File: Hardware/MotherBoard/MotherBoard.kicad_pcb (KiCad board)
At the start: 2 copper layers, 145 x 160 mm, 55 parts, among them J1 POWER, J10 I/O_PWR, J11 DMA_PULLUP, J12 NMI_PULLUP, J13 USB_OTG, J14 IRQ0_PULLUP, J2 I/O0, J3 ISA1, J4 ISA0, J5 I/O1, J6 EXTRN_CLCK, J9 Conn_02x02_Odd_Even, SW1 RESET_SW, SW2 ON_OFF, U1 AMS1117-5.0, U10 74HC245, U11 74HC245, U12 74HC245, U13 74HC541, U14 74HC541, U2 AT28C256, U3 WD65C22, U4 AS6C62256, U5 WD65C02, U6 74HC148, U7 74HC574, U8 ATF22V10B, U9 74HC245, X1 ACO-1MHz

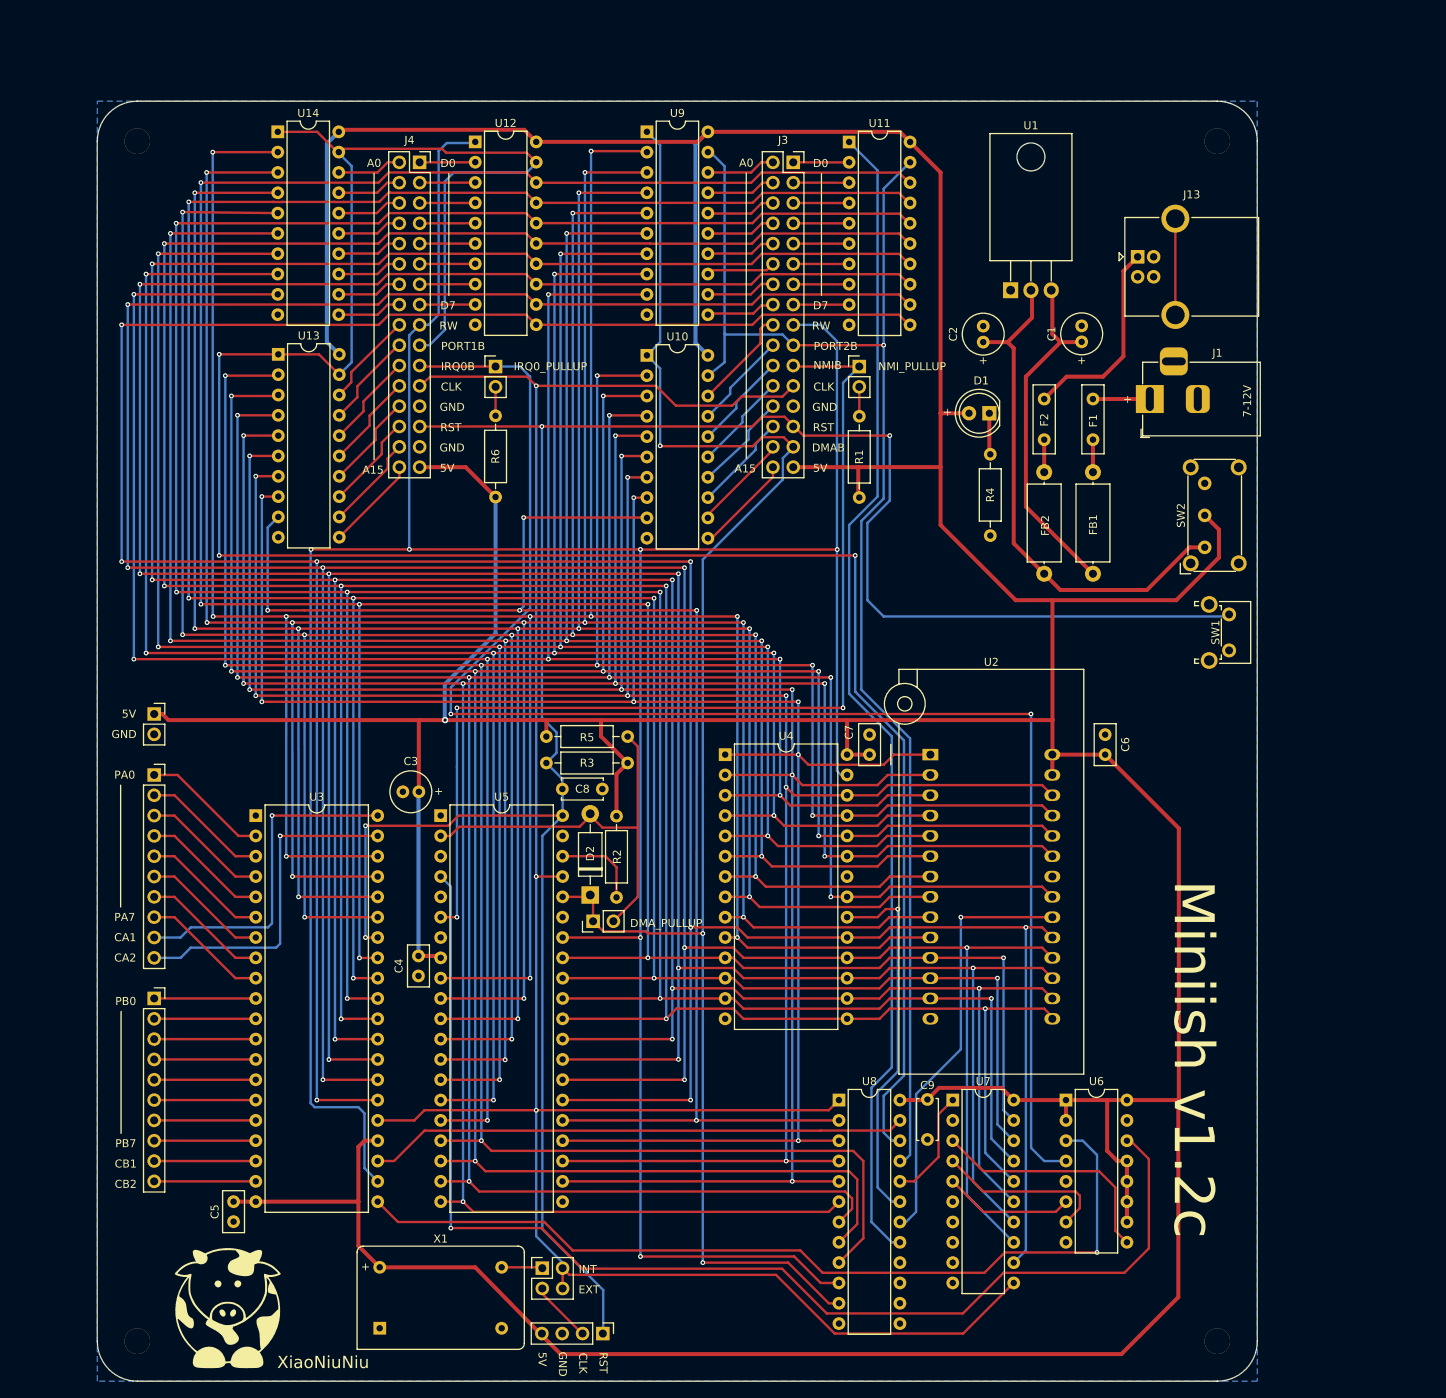
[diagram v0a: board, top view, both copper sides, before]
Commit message: New motherboard version
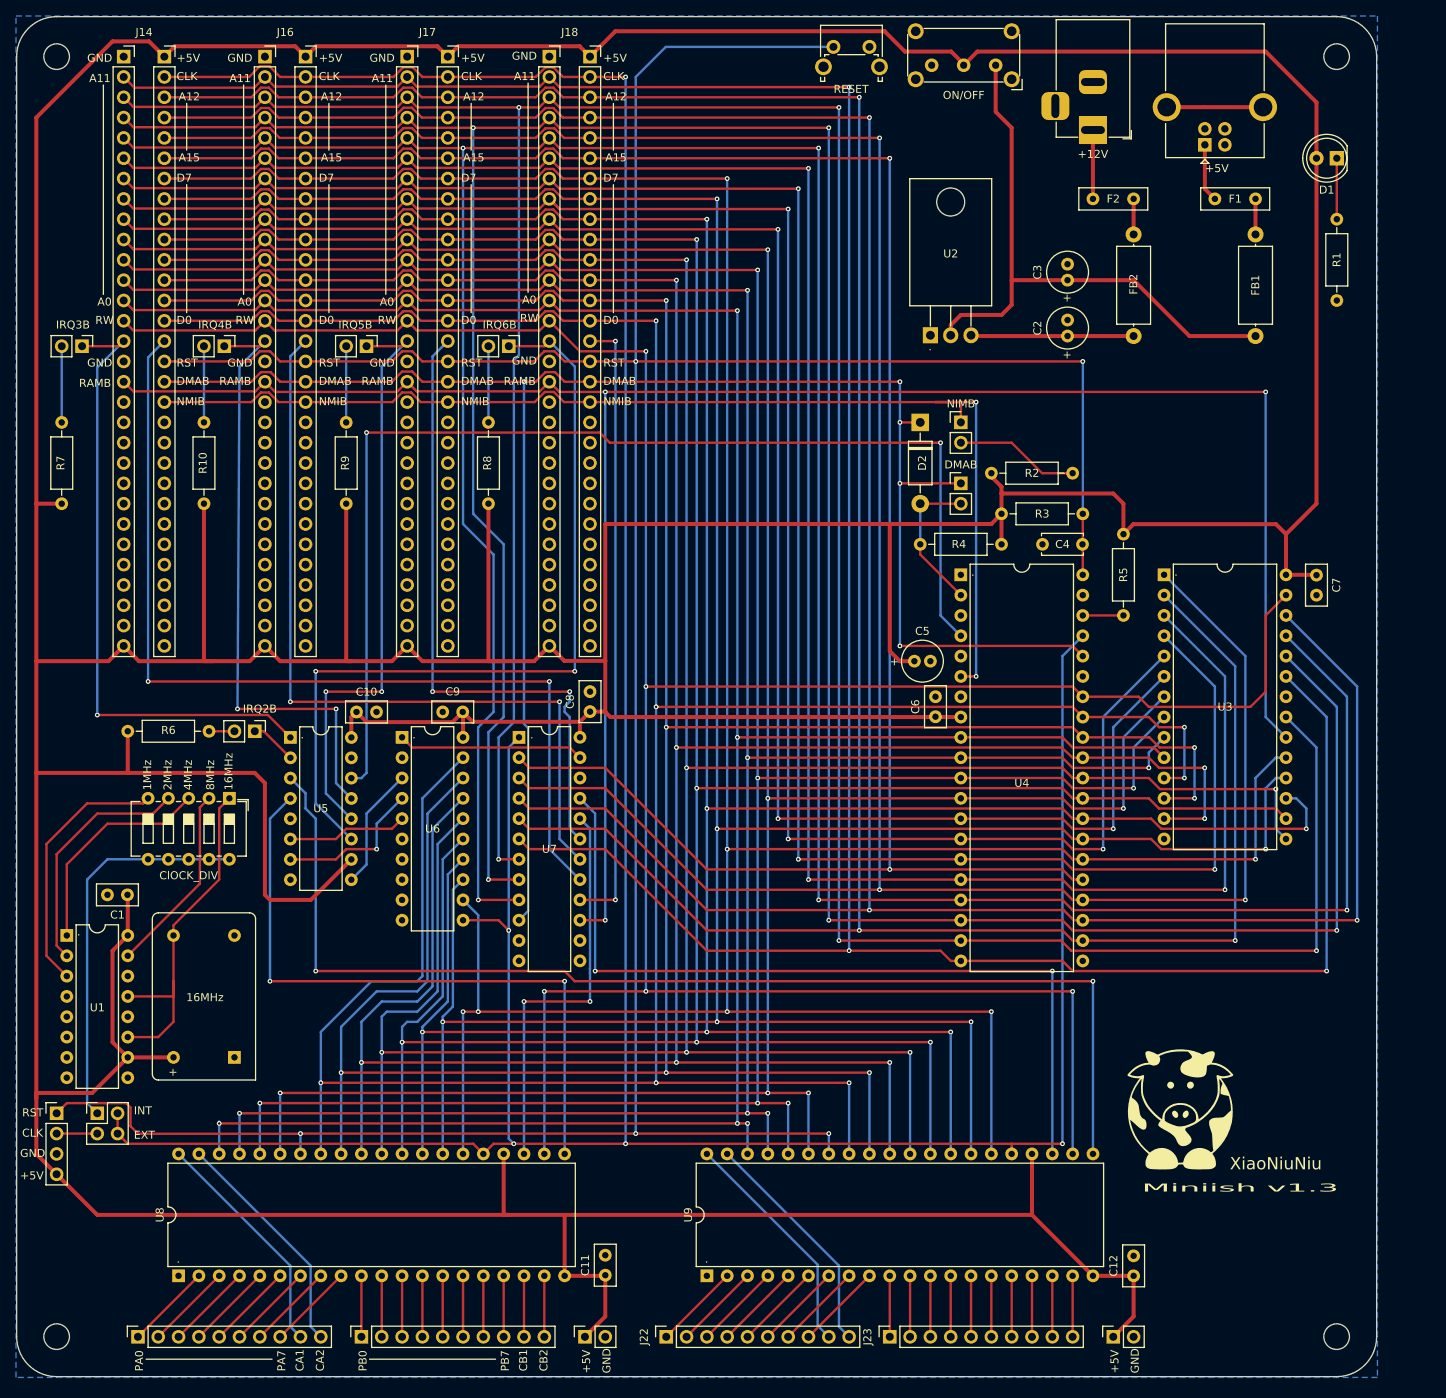
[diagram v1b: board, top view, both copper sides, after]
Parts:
- removed J1: POWER, Connector_BarrelJack:BarrelJack_Horizontal
- removed J10: I/O_PWR, Connector_PinSocket_2.54mm:PinSocket_1x02_P2.54mm_Vertical
- removed J11: DMA_PULLUP, Connector_PinHeader_2.54mm:PinHeader_1x02_P2.54mm_Vertical
- removed J12: NMI_PULLUP, Connector_PinHeader_2.54mm:PinHeader_1x02_P2.54mm_Vertical
- removed J13: USB_OTG, Connector_USB:USB_B_OST_USB-B1HSxx_Horizontal
- removed J2: I/O0, Connector_PinSocket_2.54mm:PinSocket_1x10_P2.54mm_Vertical
- removed J5: I/O1, Connector_PinSocket_2.54mm:PinSocket_1x10_P2.54mm_Vertical
- removed J6: EXTRN_CLCK, Connector_PinHeader_2.54mm:PinHeader_1x04_P2.54mm_Vertical
- removed J9: Conn_02x02_Odd_Even, Connector_PinHeader_2.54mm:PinHeader_2x02_P2.54mm_Vertical
- removed SW1: RESET_SW, Button_Switch_THT:SW_Tactile_SPST_Angled_PTS645Vx83-2LFS
- removed SW2: ON_OFF, Button_Switch_THT:SW_E-Switch_EG1224_SPDT_Angled
- removed U10, U11, U12: 74HC245, Package_DIP:DIP-20_W7.62mm
- removed U13, U14: 74HC541, Package_DIP:DIP-20_W7.62mm
- removed X1: ACO-1MHz, Oscillator:Oscillator_DIP-14
- removed the XiaoNiuNiu at (39.5, 176.1)
- added +12V: POWER, Connector_BarrelJack:BarrelJack_Horizontal, F.Cu at (147.7, 28.8)
- added +5V: USB_OTG, Connector_USB:USB_B_OST_USB-B1HSxx_Horizontal, F.Cu at (161.6, 30.7)
- added 16MHz: ACO-16MHz, Oscillator:Oscillator_DIP-14, F.Cu at (40.3, 144.7)
- added C10: 100nF, Capacitor_THT:C_Disc_D5.0mm_W2.5mm_P2.50mm, F.Cu at (55.6, 101.6)
- added C11: 100nF, Capacitor_THT:C_Disc_D5.0mm_W2.5mm_P2.50mm, F.Cu at (86.7, 172.0)
- added C12: 100nF, Capacitor_THT:C_Disc_D5.0mm_W2.5mm_P2.50mm, F.Cu at (152.7, 172.0)
- added ClOCK_DIV: CLOCK_DIV, Button_Switch_THT:SW_DIP_SPSTx05_Slide_6.7x14.26mm_W7.62mm_P2.54mm_LowProfile, F.Cu at (39.7, 112.4)
- added DMAB: DMA_PULLUP, Connector_PinHeader_2.54mm:PinHeader_1x02_P2.54mm_Vertical, F.Cu at (131.1, 73.0)
- added IRQ2B: IRQ2_PULLUP, Connector_PinHeader_2.54mm:PinHeader_1x02_P2.54mm_Vertical, F.Cu at (42.9, 104.0)
- added IRQ3B: IRQ3_PULLUP, Connector_PinHeader_2.54mm:PinHeader_1x02_P2.54mm_Vertical, F.Cu at (21.3, 55.8)
- added IRQ4B: IRQ4_PULLUP, Connector_PinHeader_2.54mm:PinHeader_1x02_P2.54mm_Vertical, F.Cu at (39.1, 55.8)
- added IRQ5B: IRQ5_PULLUP, Connector_PinHeader_2.54mm:PinHeader_1x02_P2.54mm_Vertical, F.Cu at (56.8, 55.8)
- added IRQ6B: IRQ6_PULLUP, Connector_PinHeader_2.54mm:PinHeader_1x02_P2.54mm_Vertical, F.Cu at (74.6, 55.8)
- added J16: PORT2, NESConnector:NES_Cartdrige, F.Cu at (46.7, 56.5)
- added J17: PORT2, NESConnector:NES_Cartdrige, F.Cu at (64.5, 56.5)
- added J18: PORT3, NESConnector:NES_Cartdrige, F.Cu at (82.2, 56.5)
- added J19: GPIO1, Connector_PinSocket_2.54mm:PinSocket_1x10_P2.54mm_Vertical, F.Cu at (28.3, 179.7)
- added J20: GPIO2, Connector_PinSocket_2.54mm:PinSocket_1x10_P2.54mm_Vertical, F.Cu at (56.2, 179.7)
- added J21: GPIO1_PWR, Connector_PinSocket_2.54mm:PinSocket_1x02_P2.54mm_Vertical, F.Cu at (84.2, 179.7)
- added J22: GPIO3, Connector_PinSocket_2.54mm:PinSocket_1x10_P2.54mm_Vertical, F.Cu at (94.3, 179.7)
- added J23: GPIO4, Connector_PinSocket_2.54mm:PinSocket_1x10_P2.54mm_Vertical, F.Cu at (122.2, 179.7)
- added J24: GPIO2_PWR, Connector_PinSocket_2.54mm:PinSocket_1x02_P2.54mm_Vertical, F.Cu at (150.2, 179.7)
- added NIMB: NMI_PULLUP, Connector_PinHeader_2.54mm:PinHeader_1x02_P2.54mm_Vertical, F.Cu at (131.1, 65.4)
- added ON/OFF: ON_OFF, Button_Switch_THT:SW_E-Switch_EG1224_SPDT_Angled, F.Cu at (135.5, 20.7)
- added R10: 3K3, Resistor_THT:R_Axial_DIN0207_L6.3mm_D2.5mm_P10.16mm_Horizontal, F.Cu at (36.5, 65.4)
- added R7: 3K3, Resistor_THT:R_Axial_DIN0207_L6.3mm_D2.5mm_P10.16mm_Horizontal, F.Cu at (18.7, 65.4)
- added R8: 3K3, Resistor_THT:R_Axial_DIN0207_L6.3mm_D2.5mm_P10.16mm_Horizontal, F.Cu at (72.1, 65.4)
- added R9: 3K3, Resistor_THT:R_Axial_DIN0207_L6.3mm_D2.5mm_P10.16mm_Horizontal, F.Cu at (54.3, 65.4)
- added RESET: RESET_SW, Button_Switch_THT:SW_Tactile_SPST_Angled_PTS645Vx83-2LFS, F.Cu at (115.2, 18.4)
- added XiaoNiuNiu: LOGO, Cow:SmallCow, F.Cu at (158.6, 151.2)
- C1: value 10uF -> 10nF; footprint Capacitor_THT:C_Radial_D5.0mm_H11.0mm_P2.00mm -> Capacitor_THT:C_Disc_D5.0mm_W2.5mm_P2.50mm
- C2: value 22uF -> 10uF
- C3: value 10uF -> 22uF
- C4: value 100nF -> 470nF; footprint Capacitor_THT:C_Disc_D5.0mm_W2.5mm_P2.50mm -> Capacitor_THT:C_Disc_D5.0mm_W2.5mm_P5.00mm
- C5: value 100nF -> 10uF; footprint Capacitor_THT:C_Disc_D5.0mm_W2.5mm_P2.50mm -> Capacitor_THT:C_Radial_D5.0mm_H11.0mm_P2.00mm
- C8: value 470nF -> 220nF; footprint Capacitor_THT:C_Disc_D5.0mm_W2.5mm_P5.00mm -> Capacitor_THT:C_Disc_D5.0mm_W2.5mm_P2.50mm
- C9: value 220nF -> 100nF; footprint Capacitor_THT:C_Disc_D5.0mm_W2.5mm_P5.00mm -> Capacitor_THT:C_Disc_D5.0mm_W2.5mm_P2.50mm
- J14: value IRQ0_PULLUP -> PORT1; footprint Connector_PinHeader_2.54mm:PinHeader_1x02_P2.54mm_Vertical -> NESConnector:NES_Cartdrige
- J3: value ISA1 -> CLOCK_SEL; footprint Connector_PinSocket_2.54mm:PinSocket_2x16_P2.54mm_Vertical -> Connector_PinHeader_2.54mm:PinHeader_2x02_P2.54mm_Vertical
- J4: value ISA0 -> EXTRN_CLCK; footprint Connector_PinSocket_2.54mm:PinSocket_2x16_P2.54mm_Vertical -> Connector_PinHeader_2.54mm:PinHeader_1x04_P2.54mm_Vertical
- R1: value 3K3 -> 220
- R4: value 220 -> 3K3
- U1: value AMS1117-5.0 -> 74HC590A; footprint Package_TO_SOT_THT:TO-220-3_Horizontal_TabDown -> Package_DIP:DIP-16_W7.62mm
- U2: value AT28C256 -> AMS1117-5.0; footprint Socket:DIP_Socket-28_W11.9_W12.7_W15.24_W17.78_W18.5_3M_228-1277-00-0602J -> Package_TO_SOT_THT:TO-220-3_Horizontal_TabDown
- U3: value WD65C22 -> AS6C62256; footprint Package_DIP:DIP-40_W15.24mm -> Package_DIP:DIP-28_W15.24mm
- U4: value AS6C62256 -> WD65C02; footprint Package_DIP:DIP-28_W15.24mm -> Package_DIP:DIP-40_W15.24mm
- U5: value WD65C02 -> 74HC148; footprint Package_DIP:DIP-40_W15.24mm -> Package_DIP:DIP-16_W7.62mm
- U6: value 74HC148 -> 74HC574; footprint Package_DIP:DIP-16_W7.62mm -> Package_DIP:DIP-20_W7.62mm
- U7: value 74HC574 -> ATF22V10B; footprint Package_DIP:DIP-20_W7.62mm -> Package_DIP:DIP-24_W7.62mm
- U8: value ATF22V10B -> WD65C22; footprint Package_DIP:DIP-24_W7.62mm -> Package_DIP:DIP-40_W15.24mm
- U9: value 74HC245 -> WD65C22; footprint Package_DIP:DIP-20_W7.62mm -> Package_DIP:DIP-40_W15.24mm
- moved H2 150.3 mm to (178.1, 19.6)
- moved H3 149.9 mm to (178.1, 179.6)
- moved J3 147.3 mm to (23.2, 151.7)
- moved H1 145.5 mm to (18.1, 19.6)
- moved H4 145.1 mm to (18.1, 179.6)
- moved U9 143.2 mm to (99.4, 172.0), turned to 90 degrees
- moved U1 142.9 mm to (19.4, 129.5)
- moved C1 137.9 mm to (27.0, 124.4), turned to 180 degrees
- moved J4 127.2 mm to (18.1, 151.7)
- moved U3 117.5 mm to (156.5, 84.4)
- moved C5 108.7 mm to (125.3, 95.2), turned to 0 degrees
- moved C3 103.3 mm to (144.5, 47.6), turned to 90 degrees
- moved C4 97.7 mm to (146.3, 80.6), turned to 180 degrees
- moved U6 94.6 mm to (61.3, 104.7)
- moved U8 85.4 mm to (33.4, 172.0), turned to 90 degrees
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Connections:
- C1 pad 1: Net-(C1-Pad1) -> +5V
- C2 pad 1: Net-(C2-Pad1) -> Net-(#FLG01-pwr)
- C3 pad 1: +5V -> Net-(SW2-A)
- C4 pad 1: +5V -> RESET
- C8 pad 1: RESET -> +5V
- D1 pad 1: Net-(D1-Pad1) -> Net-(D1-K)
- D2 pad 1: /Main /DMAB -> /North Bridge/DMAB
- D2 pad 2: /Main /RDY -> /North Bridge/RDY
- FB1 pad 2: Net-(C1-Pad1) -> Net-(SW2-A)
- FB2 pad 2: Net-(C2-Pad1) -> Net-(#FLG01-pwr)
- J14 pad 1: /North Bridge/IRQ0B -> GND
- J14 pad 2: Net-(J14-Pad2) -> +5V
- J3 pad 2: Net-(J3-Pad2) -> CLOCK
- J3 pad 3: Net-(J3-Pad3) -> ECLOCK
- J3 pad 4: Net-(J3-Pad4) -> CLOCK
- J4 pad 1: Net-(J4-Pad1) -> RESET
- J4 pad 2: Net-(J4-Pad2) -> ECLOCK
- J4 pad 3: Net-(J4-Pad3) -> GND
- J4 pad 4: Net-(J4-Pad4) -> +5V
- R1 pad 1: Net-(J12-Pad2) -> Net-(D1-K)
- R1 pad 2: +5V -> GND
- R2 pad 1: +5V -> Net-(J5-Pin_2)
- R2 pad 2: Net-(R2-Pad2) -> +5V
- R4 pad 1: Net-(D1-Pad1) -> /North Bridge/RDY
- R4 pad 2: GND -> +5V
- R5 pad 1: /Main /RDY -> +5V
- R5 pad 2: +5V -> /North Bridge/SOB
- R6 pad 1: Net-(J14-Pad2) -> Net-(J7-Pin_2)
- U1 pad 1: GND -> /4MHz
- U1 pad 2: Net-(C2-Pad1) -> /2MHz
- U1 pad 3: Net-(C1-Pad1) -> /1MHz
- U2 pad 1: /A14 -> GND
- U2 pad 2: /A12 -> Net-(SW2-A)
- U2 pad 3: /A7 -> Net-(#FLG01-pwr)
- U3 pad 1: GND -> /GPIO/A14
- U3 pad 10: PB0 -> /GPIO/A0
- U3 pad 11: PB1 -> /GPIO/D0
- U3 pad 12: PB2 -> /GPIO/D1
- U3 pad 13: PB3 -> /GPIO/D2
- U3 pad 14: PB4 -> GND
- U3 pad 15: PB5 -> /GPIO/D3
- U3 pad 16: PB6 -> /GPIO/D4
- U3 pad 17: PB7 -> /GPIO/D5
- U3 pad 18: CB1 -> /GPIO/D6
- U3 pad 19: CB2 -> /GPIO/D7
- U3 pad 2: PA0 -> /GPIO/A12
- U3 pad 20: +5V -> /North Bridge/RAMCSB
- U3 pad 21: /Main /IRQ1B -> /GPIO/A10
- U3 pad 22: /Main /RW -> GND
- U3 pad 23: /Main /IOCSB -> /GPIO/A11
- U3 pad 24: +5V -> /GPIO/A9
- U3 pad 25: CLOCK -> /GPIO/A8
- U3 pad 26: /D7 -> /GPIO/A13
- U3 pad 27: /D6 -> /GPIO/RW
- U3 pad 28: /D5 -> +5V
- U3 pad 3: PA1 -> /GPIO/A7
- U3 pad 4: PA2 -> /GPIO/A6
- U3 pad 5: PA3 -> /GPIO/A5
- U3 pad 6: PA4 -> /GPIO/A4
- U3 pad 7: PA5 -> /GPIO/A3
- U3 pad 8: PA6 -> /GPIO/A2
- U3 pad 9: PA7 -> /GPIO/A1
- U4 pad 1: /A14 -> unconnected-(U4-~{VP}-Pad1)
- U4 pad 10: /A0 -> /GPIO/A1
- U4 pad 11: /D0 -> /GPIO/A2
- U4 pad 12: /D1 -> /GPIO/A3
- U4 pad 13: /D2 -> /GPIO/A4
- U4 pad 14: GND -> /GPIO/A5
- U4 pad 15: /D3 -> /GPIO/A6
- U4 pad 16: /D4 -> /GPIO/A7
- U4 pad 17: /D5 -> /GPIO/A8
- U4 pad 18: /D6 -> /GPIO/A9
- U4 pad 19: /D7 -> /GPIO/A10
- U4 pad 2: /A12 -> /North Bridge/RDY
- U4 pad 20: /Main /RAMCSB -> /GPIO/A11
- U4 pad 21: /A10 -> GND
- U4 pad 22: GND -> /GPIO/A12
- U4 pad 23: /A11 -> /GPIO/A13
- U4 pad 24: /A9 -> /GPIO/A14
- U4 pad 25: /A8 -> /GPIO/A15
- U4 pad 26: /A13 -> /GPIO/D7
- U4 pad 27: /Main /RW -> /GPIO/D6
- U4 pad 28: +5V -> /GPIO/D5
- U4 pad 3: /A7 -> unconnected-(U4-PHI1out-Pad3)
- U4 pad 4: /A6 -> /North Bridge/IRQB
- U4 pad 5: /A5 -> unconnected-(U4-~{ML}-Pad5)
- U4 pad 6: /A4 -> /North Bridge/NMIB
- U4 pad 7: /A3 -> unconnected-(U4-SYNC-Pad7)
- U4 pad 8: /A2 -> +5V
- U4 pad 9: /A1 -> /GPIO/A0
- U5 pad 1: unconnected-(U5-Pad1) -> /Ports/IRQ3B
- U5 pad 10: /A1 -> +5V
- U5 pad 11: /A2 -> /Ports/IRQ6B
- U5 pad 12: /A3 -> /Ports/IRQ5B
- U5 pad 13: /A4 -> /Ports/IRQ4B
- U5 pad 14: /A5 -> /North Bridge/IRQB
- U5 pad 15: /A6 -> unconnected-(U5-EO-Pad15)
- U5 pad 16: /A7 -> +5V
- U5 pad 2: /Main /RDY -> /Ports/IRQ2B
- U5 pad 3: unconnected-(U5-Pad3) -> /GPIO/IRQ1B
- U5 pad 4: /Main /IRQB -> /GPIO/IRQ0B
- U5 pad 5: unconnected-(U5-Pad5) -> GND
- U5 pad 6: /Main /NMIB -> Net-(U5-S2)
- U5 pad 7: unconnected-(U5-Pad7) -> Net-(U5-S1)
- U5 pad 8: +5V -> GND
- U5 pad 9: /A0 -> Net-(U5-S0)
- U6 pad 1: +5V -> Net-(U6-OE)
- U6 pad 10: +5V -> GND
- U6 pad 11: +5V -> CLOCK
- U6 pad 12: +5V -> /GPIO/D7
- U6 pad 13: +5V -> /GPIO/D6
- U6 pad 14: /Main /IRQB -> /GPIO/D5
- U6 pad 15: unconnected-(U6-Pad15) -> /GPIO/D4
- U6 pad 16: +5V -> /GPIO/D3
- U6 pad 2: +5V -> GND
- U6 pad 3: /Main /IRQ1B -> Net-(U5-S0)
- U6 pad 4: /North Bridge/IRQ0B -> Net-(U5-S1)
- U6 pad 5: GND -> Net-(U5-S2)
- U6 pad 6: Net-(U6-Pad6) -> GND
- U6 pad 7: Net-(U6-Pad7) -> GND
- U6 pad 9: Net-(U6-Pad9) -> GND
- U7 pad 1: Net-(U7-Pad1) -> CLOCK
- U7 pad 10: GND -> /North Bridge/DMAB
- U7 pad 11: CLOCK -> GND
- U7 pad 12: /D7 -> GND
- U7 pad 13: /D6 -> GND
- U7 pad 14: /D5 -> unconnected-(U7-O9-Pad14)
- U7 pad 15: /D4 -> /North Bridge/RAMCSB
- U7 pad 16: /D3 -> /Ports/ROMCSB
- U7 pad 17: /D2 -> /Ports/PORT1CSB
- U7 pad 18: /D1 -> /Ports/PORT2CSB
- U7 pad 19: /D0 -> /Ports/PORT3CSB
- U7 pad 2: GND -> /GPIO/A15
- U7 pad 20: +5V -> /GPIO/CIA1CSB
- U7 pad 3: Net-(U6-Pad9) -> /GPIO/A14
- U7 pad 4: Net-(U6-Pad7) -> /GPIO/A13
- U7 pad 5: Net-(U6-Pad6) -> /GPIO/A12
- U7 pad 6: GND -> /GPIO/A11
- U7 pad 7: GND -> /GPIO/A10
- U7 pad 8: GND -> /GPIO/A9
- U7 pad 9: GND -> /GPIO/A8
- U8 pad 1: CLOCK -> GND
- U8 pad 10: /Main /RW -> PB10
- U8 pad 11: /Main /DMAB -> PB11
- U8 pad 12: GND -> PB12
- U8 pad 13: GND -> PB13
- U8 pad 14: unconnected-(U8-Pad14) -> PB14
- U8 pad 15: unconnected-(U8-Pad15) -> PB15
- U8 pad 16: unconnected-(U8-Pad16) -> PB16
- U8 pad 17: /North Bridge/DMARW -> PB17
- U8 pad 18: /Main /ROMCSB -> CB11
- U8 pad 19: /Main /RAMCSB -> CB12
- U8 pad 2: /A15 -> PA10
- U8 pad 20: Net-(U7-Pad1) -> +5V
- U8 pad 21: /North Bridge/PORT2B -> /GPIO/IRQ0B
- U8 pad 22: /North Bridge/PORT1B -> /GPIO/RW
- U8 pad 23: /Main /IOCSB -> /GPIO/CIA1CSB
- U8 pad 3: /A14 -> PA11
- U8 pad 4: /A13 -> PA12
- U8 pad 5: /A12 -> PA13
- U8 pad 6: /A11 -> PA14
- U8 pad 7: /A10 -> PA15
- U8 pad 8: /A9 -> PA16
- U8 pad 9: /A8 -> PA17
- U9 pad 1: /Main /DMAB -> GND
- U9 pad 10: GND -> PB20
- U9 pad 11: Net-(J3-Pad24) -> PB21
- U9 pad 12: Net-(J3-Pad23) -> PB22
- U9 pad 13: Net-(J3-Pad22) -> PB23
- U9 pad 14: Net-(J3-Pad21) -> PB24
- U9 pad 15: Net-(J3-Pad20) -> PB25
- U9 pad 16: Net-(J3-Pad19) -> PB26
- U9 pad 17: Net-(J3-Pad18) -> PB27
- U9 pad 18: Net-(J3-Pad17) -> CB21
- U9 pad 19: /North Bridge/PORT2B -> CB22
- U9 pad 2: /A0 -> PA20
- U9 pad 3: /A1 -> PA21
- U9 pad 4: /A2 -> PA22
- U9 pad 5: /A3 -> PA23
- U9 pad 6: /A4 -> PA24
- U9 pad 7: /A5 -> PA25
- U9 pad 8: /A6 -> PA26
- U9 pad 9: /A7 -> PA27
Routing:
- net /D7: track 448.8 -> 0.00 mm, vias 8 -> 0
- net /D6: track 439.1 -> 0.00 mm, vias 8 -> 0
- net /D5: track 426.1 -> 0.00 mm, vias 8 -> 0
- net /D4: track 412.6 -> 0.00 mm, vias 8 -> 0
- net /D3: track 399.8 -> 0.00 mm, vias 7 -> 0
- net /Main /RW: track 393.4 -> 0.00 mm, vias 6 -> 0
- net /GPIO/A9: track 0.00 -> 391.9 mm, vias 0 -> 5
- net /GPIO/A8: track 0.00 -> 389.9 mm, vias 0 -> 5
- net /GPIO/A10: track 0.00 -> 385.7 mm, vias 0 -> 5
- net /D2: track 381.7 -> 0.00 mm, vias 7 -> 0
- net /GPIO/D3: track 0.00 -> 375.9 mm, vias 0 -> 6
- net /GPIO/D7: track 0.00 -> 375.4 mm, vias 0 -> 7
- net /D1: track 374.4 -> 0.00 mm, vias 7 -> 0
- net /GPIO/D5: track 0.00 -> 374.2 mm, vias 0 -> 6
- net /GPIO/D6: track 0.00 -> 373.2 mm, vias 0 -> 6
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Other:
- board size 145 x 160 mm -> 170 x 170 mm
- board text added: "+5V"
- board text added: "."
- board text added: "16MHz"
- board text added: "1MHz"
- board text added: "2MHz"
- board text added: "4MHz"
- board text added: "8MHz"
- board text added: "A11"
- board text added: "A12"
- board text added: "Miniish v1.3"
- board text added: "RAMB"
- board text removed: "5V"
- board text removed: "7-12V"
- board text removed: "IRQ0B"
- board text removed: "Miniish v1.2c"
- board text removed: "PORT1B"
- board text removed: "PORT2B"
